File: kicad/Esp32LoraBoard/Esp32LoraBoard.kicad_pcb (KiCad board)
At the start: 2 copper layers, 71.8 x 64.1 mm, 53 parts, among them J1 USB_B_Micro, J2 Power-Selector, J3 Testpoints, J4 ESP_PROG_JTAG, J5 Prog, J6 ext_Measure, J7 Measurement-Selector, J8 OLED_128x64, Q1 UMH3N, Q2 Si2302DS_NMOS, Q3 Si2301DS_PMOS, Q4 Si2302DS_NMOS, Q5 Si2301DS_PMOS, Q6 Si2302DS_NMOS, SW1 Rotary_Encoder, SW2 Reset, U1 LM3940IMP-3.3, U2 ESP32-WROOM-32, U3 RFM95W-868S2

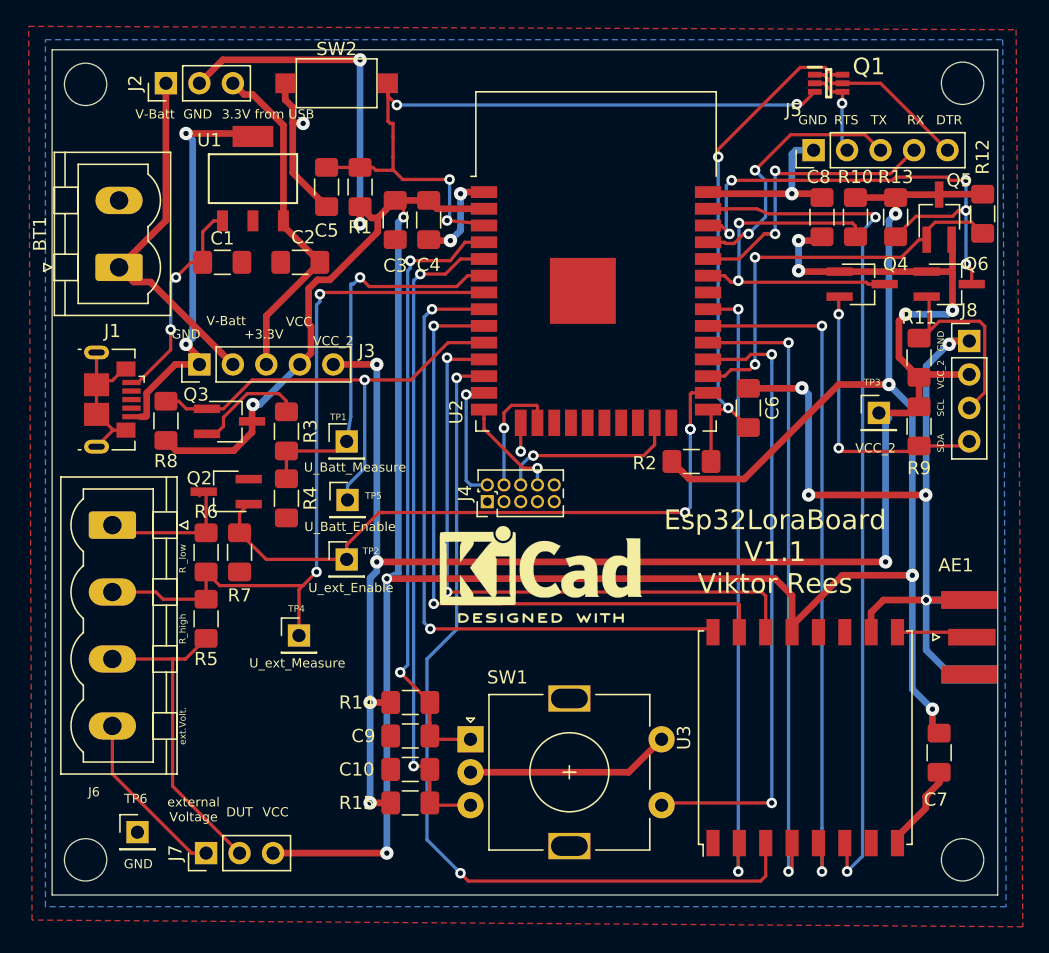
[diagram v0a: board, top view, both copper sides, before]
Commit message: new PCB Version V1.2
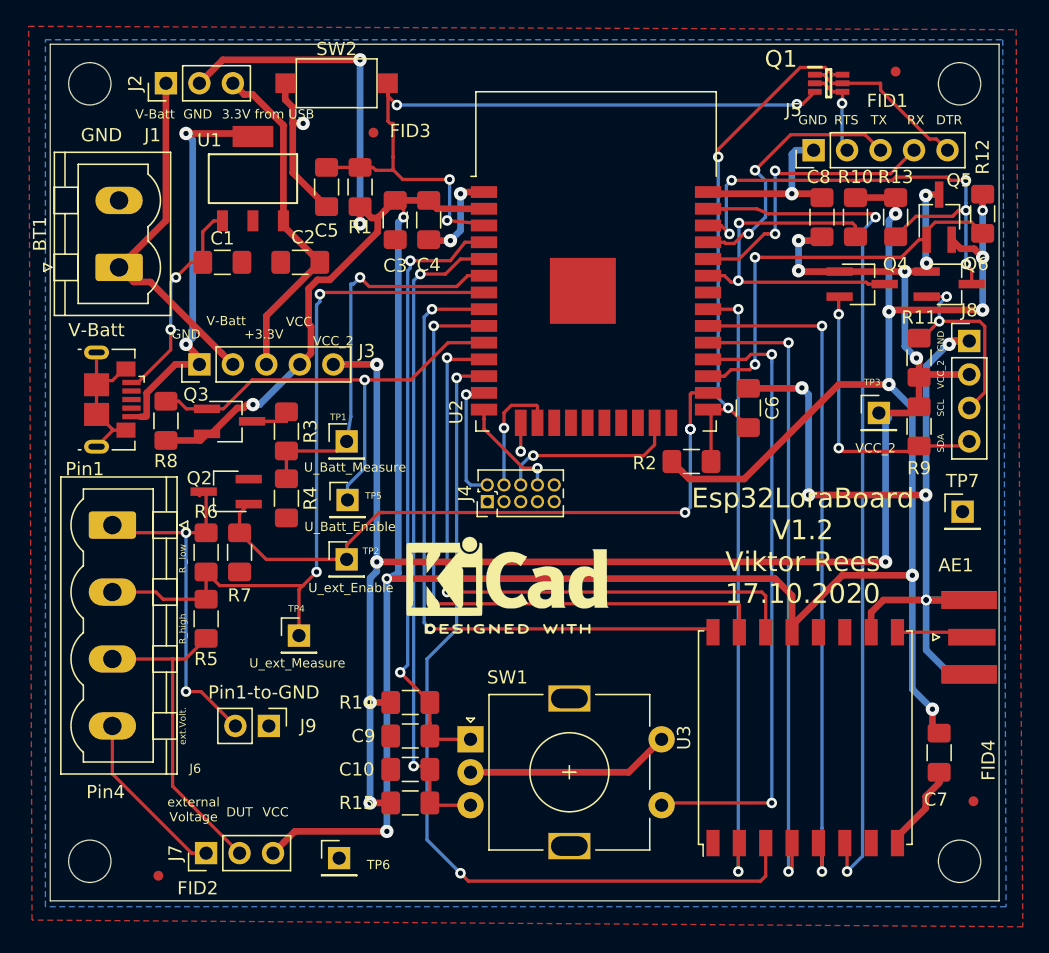
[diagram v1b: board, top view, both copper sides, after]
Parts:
- added FID1: Fiducial, Fiducial:Fiducial_0.75mm_Mask1.5mm, F.Cu at (168.1, 60.1)
- added FID2: Fiducial, Fiducial:Fiducial_0.75mm_Mask1.5mm, F.Cu at (112.2, 121.1)
- added FID3: Fiducial, Fiducial:Fiducial_0.75mm_Mask1.5mm, F.Cu at (128.5, 64.7)
- added FID4: Fiducial, Fiducial:Fiducial_0.75mm_Mask1.5mm, F.Cu at (174.1, 115.4)
- added J9: Pin1-to-GND, Connector_PinHeader_2.54mm:PinHeader_1x02_P2.54mm_Vertical, F.Cu at (120.6, 109.7)
- added TP7: GND, Connector_PinHeader_2.54mm:PinHeader_1x01_P2.54mm_Vertical, F.Cu at (173.2, 93.5)
- moved TP6 15.4 mm to (125.9, 119.8)
- moved REF** 2.67 mm to (138.7, 98.4)
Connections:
- Q3 pad 2: Net-(Q3-Pad2) -> VCC
- Q3 pad 3: VCC -> Net-(Q3-Pad3)
- Q5 pad 2: /VCC_2 -> VCC
- Q5 pad 3: VCC -> /VCC_2
- R3 pad 1: Net-(Q3-Pad2) -> Net-(Q3-Pad3)
- U2 pad 39: (no net) -> GND
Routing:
- net Net-(J6-Pad1): track 10.6 -> 27.5 mm, vias 0 -> 2
- net VCC: track 243.1 -> 253.6 mm, vias 10 -> 14
- net Net-(Q3-Pad2): track 8.73 -> 0.00 mm
- net Net-(Q3-Pad3): track 0.00 -> 3.33 mm
- net /SCL_2: track 14.1 -> 15.3 mm, vias 0 -> 2
- net /VCC_2: track 130.0 -> 129.0 mm, vias 9 -> 11
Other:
- board size 71.8 x 64.1 mm -> 72 x 65 mm
- board text added: "Esp32LoraBoard V1.2 Viktor Rees 17.10.2020"
- board text added: "Pin1"
- board text added: "Pin1-to-GND"
- board text added: "Pin4"
- board text removed: "Esp32LoraBoard V1.1 Viktor Rees"
